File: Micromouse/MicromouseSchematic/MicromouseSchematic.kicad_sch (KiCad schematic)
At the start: 28 parts, among them J10 Conn_01x06_MountingPin, J3 Conn_01x04_Pin, J4 Conn_01x02_Pin, J5 Conn_01x06_MountingPin, SW1 SW_Push, SW2 SW_Push, U5 STM32F746VETx, Y1 8MHz, Y2 32.768kHz

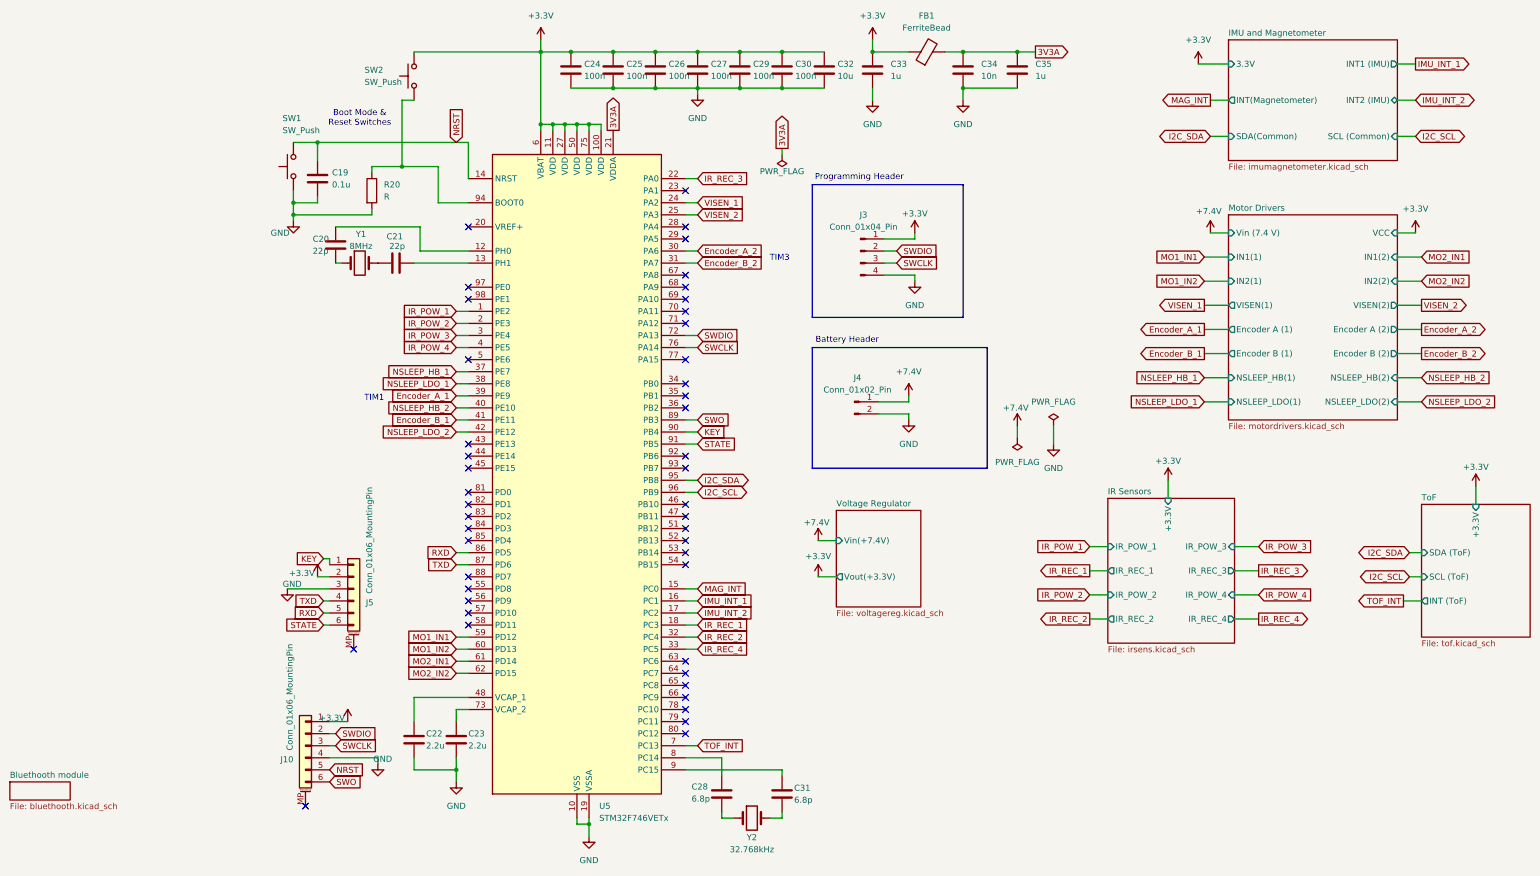
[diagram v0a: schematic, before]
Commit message: udpated programming header
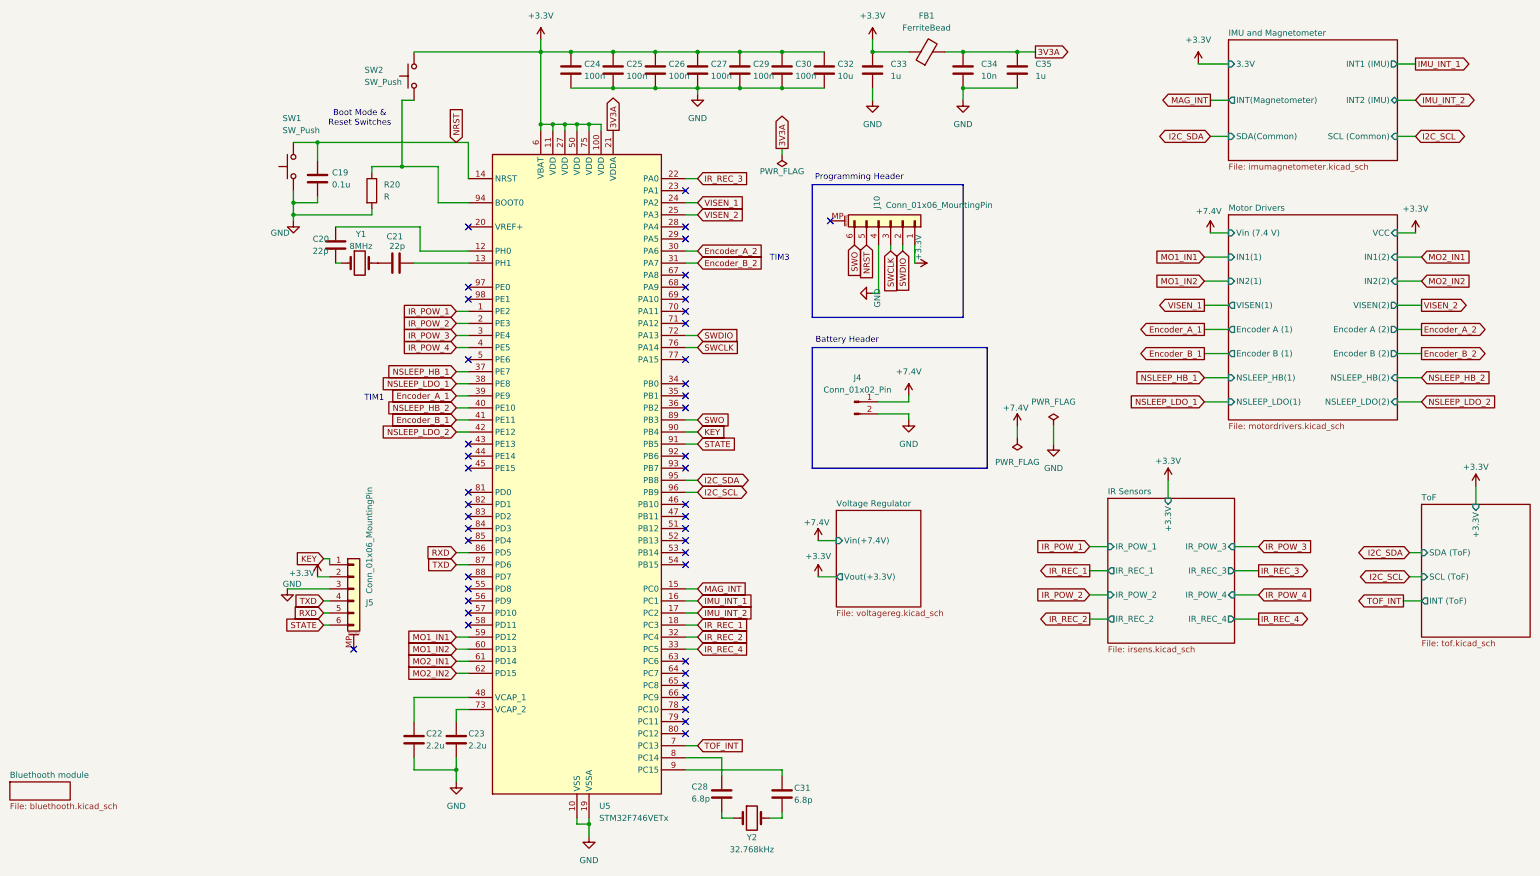
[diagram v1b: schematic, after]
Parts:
- removed J3: Conn_01x04_Pin, symbol Connector:Conn_01x04_Pin
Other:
- moved on the sheet: J10
